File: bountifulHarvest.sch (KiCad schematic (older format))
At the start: 0 parts

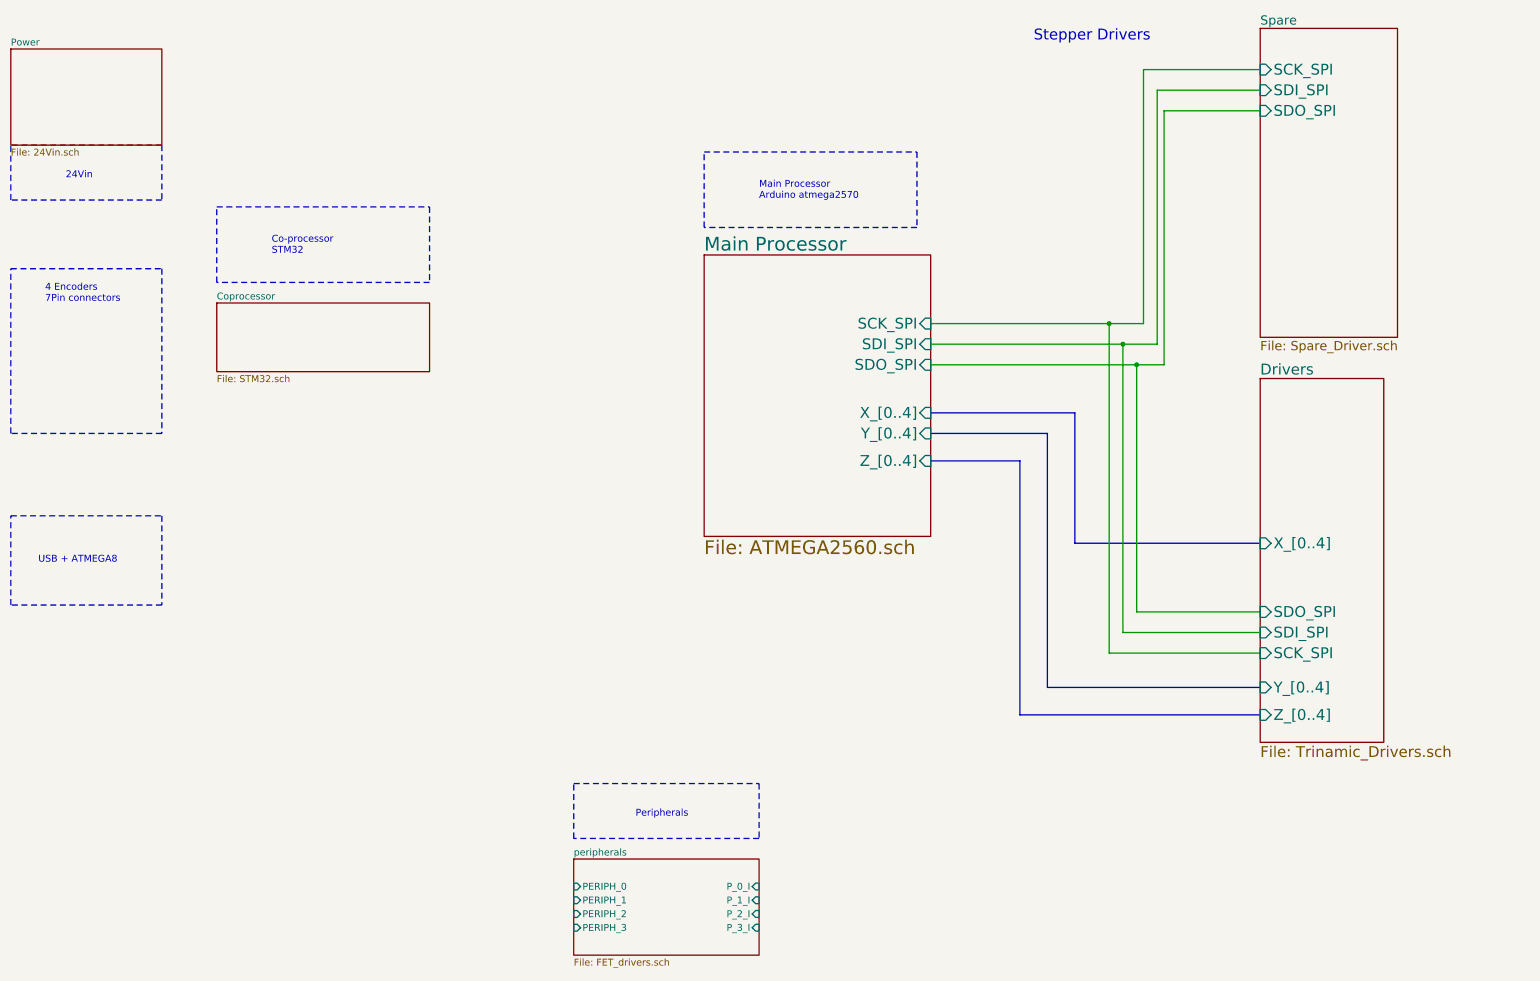
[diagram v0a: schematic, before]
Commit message: added peripherals
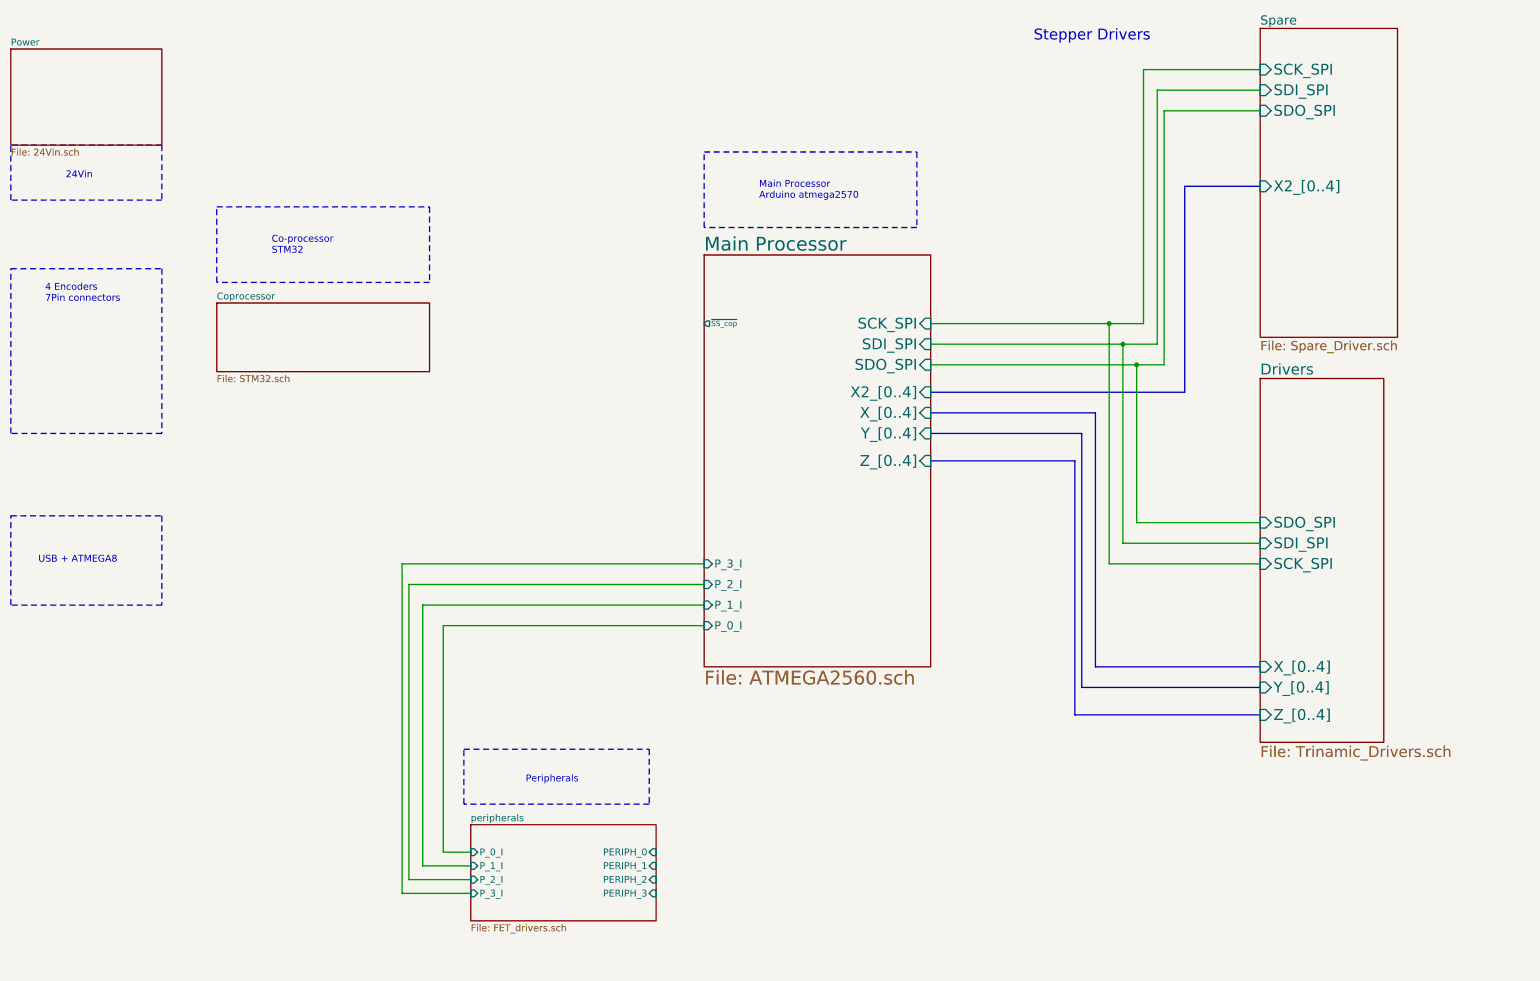
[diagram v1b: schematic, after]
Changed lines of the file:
@@
 $EndSheet
 Wire Notes Line
-	5100 6150 6450 6150
+	4300 5900 5650 5900
 Wire Notes Line
 	1000 4200 2100 4200
@@
 Stepper Drivers
 $Sheet
-S 5100 6700 1350 700
+S 4350 6450 1350 700
 U 5F08C095
 F0 "peripherals" 50
 F1 "FET_drivers.sch" 50
-F2 "PERIPH_0" I L 5100 6900 50
-F3 "PERIPH_1" I L 5100 7000 50
-F4 "PERIPH_2" I L 5100 7100 50
-F5 "PERIPH_3" I L 5100 7200 50
-F6 "P_0_I" I R 6450 6900 50
-F7 "P_3_I" I R 6450 7200 50
-F8 "P_1_I" I R 6450 7000 50
-F9 "P_2_I" I R 6450 7100 50
+F2 "PERIPH_0" I R 5700 6650 50
+F3 "PERIPH_1" I R 5700 6750 50
+F4 "PERIPH_2" I R 5700 6850 50
+F5 "PERIPH_3" I R 5700 6950 50
+F6 "P_0_I" I L 4350 6650 50
+F7 "P_3_I" I L 4350 6950 50
+F8 "P_1_I" I L 4350 6750 50
+F9 "P_2_I" I L 4350 6850 50
 $EndSheet
-Text Notes 5550 6400 0    50   ~ 0
+Text Notes 4750 6150 0    50   ~ 0
 Peripherals\n
 Wire Notes Line
-	5100 6550 5100 6150
+	4300 6300 4300 5900
 Wire Notes Line
-	6450 6550 5100 6550
+	5650 6300 4300 6300
 Wire Notes Line
-	6450 6150 6450 6550
+	5650 5900 5650 6300
 $Sheet
-S 6050 2300 1650 2050
+S 6050 2300 1650 3000
 U 5EE66603
 F0 "Main Processor" 100
@@
 F6 "Y_[0..4]" I R 7700 3600 79
 F7 "Z_[0..4]" I R 7700 3800 79
+F8 "~SS_cop" O L 6050 2800 39
+F9 "X2_[0..4]" I R 7700 3300 79
+F10 "P_0_I" I L 6050 5000 59
+F11 "P_1_I" I L 6050 4850 59
+F12 "P_2_I" I L 6050 4700 59
+F13 "P_3_I" I L 6050 4550 59
 $EndSheet
 Wire Wire Line
@@
 	9400 1250 10100 1250
 Wire Wire Line
-	10100 5200 9000 5200
+	10100 4550 9000 4550
 Wire Wire Line
-	9000 5200 9000 2800
+	9000 4550 9000 2800
 Connection ~ 9000 2800
 Wire Wire Line
 	9000 2800 7700 2800
 Wire Wire Line
-	10100 5050 9100 5050
+	10100 4400 9100 4400
 Wire Wire Line
-	9100 5050 9100 2950
+	9100 4400 9100 2950
 Connection ~ 9100 2950
 Wire Wire Line
 	9100 2950 7700 2950
 Wire Wire Line
-	10100 4900 9200 4900
+	10100 4250 9200 4250
 Wire Wire Line
-	9200 4900 9200 3100
+	9200 4250 9200 3100
 Connection ~ 9200 3100
 Wire Wire Line
 	9200 3100 9400 3100
 Wire Bus Line
-	10100 4400 8750 4400
+	10100 5300 8900 5300
 Wire Bus Line
-	8750 4400 8750 3450
+	8900 5300 8900 3450
 Wire Bus Line
-	10100 5450 8550 5450
+	10100 5450 8800 5450
 Wire Bus Line
-	8550 5450 8550 3600
+	8800 5450 8800 3600
 Wire Bus Line
-	8550 3600 7700 3600
+	8800 3600 7700 3600
 Wire Bus Line
-	10100 5650 8350 5650
+	10100 5650 8750 5650
 Wire Bus Line
-	8350 5650 8350 3800
+	8750 5650 8750 3800
 Wire Bus Line
-	8350 3800 7700 3800
+	8750 3800 7700 3800
 $Sheet
 S 10100 3200 900  2650
@@
 F0 "Drivers" 79
 F1 "Trinamic_Drivers.sch" 79
-F2 "SDO_SPI" I L 10100 4900 79
-F3 "SDI_SPI" I L 10100 5050 79
-F4 "SCK_SPI" I L 10100 5200 79
-F5 "X_[0..4]" I L 10100 4400 79
+F2 "SDO_SPI" I L 10100 4250 79
+F3 "SDI_SPI" I L 10100 4400 79
+F4 "SCK_SPI" I L 10100 4550 79
+F5 "X_[0..4]" I L 10100 5300 79
 F6 "Y_[0..4]" I L 10100 5450 79
 F7 "Z_[0..4]" I L 10100 5650 79
 $EndSheet
 Wire Bus Line
-	7700 3450 8750 3450
+	7700 3450 8900 3450
 $Sheet
 S 10100 650  1000 2250
@@
 F3 "SDI_SPI" I L 10100 1100 79
 F4 "SDO_SPI" I L 10100 1250 79
+F5 "X2_[0..4]" I L 10100 1800 79
 $EndSheet
+Wire Bus Line
+	9550 3300 9550 1800
+Wire Bus Line
+	9550 1800 10100 1800
+Wire Bus Line
+	7700 3300 9550 3300
+Wire Wire Line
+	6050 5000 4150 5000
+Wire Wire Line
+	4150 5000 4150 6650
+Wire Wire Line
+	4150 6650 4350 6650
+Wire Wire Line
+	4350 6750 4000 6750
+Wire Wire Line
+	4000 6750 4000 4850
+Wire Wire Line
+	4000 4850 6050 4850
+Wire Wire Line
+	6050 4700 3900 4700
+Wire Wire Line
+	3900 4700 3900 6850
+Wire Wire Line
+	3900 6850 4350 6850
+Wire Wire Line
+	6050 4550 3850 4550
+Wire Wire Line
+	3850 4550 3850 6950
+Wire Wire Line
+	3850 6950 4350 6950
 $EndSCHEMATC
